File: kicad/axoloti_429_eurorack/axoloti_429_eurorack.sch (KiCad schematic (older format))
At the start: 11 parts, among them J1 SERIAL_SYSTEM_BOOTLOADER, J11 I2C1_HEADER, J30 429_Conn_02x27_Odd_Even_mirro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, J8 429_Conn_02x27_Odd_Even, SW1 BOOT_FLASH, U2 STM32F427IITx

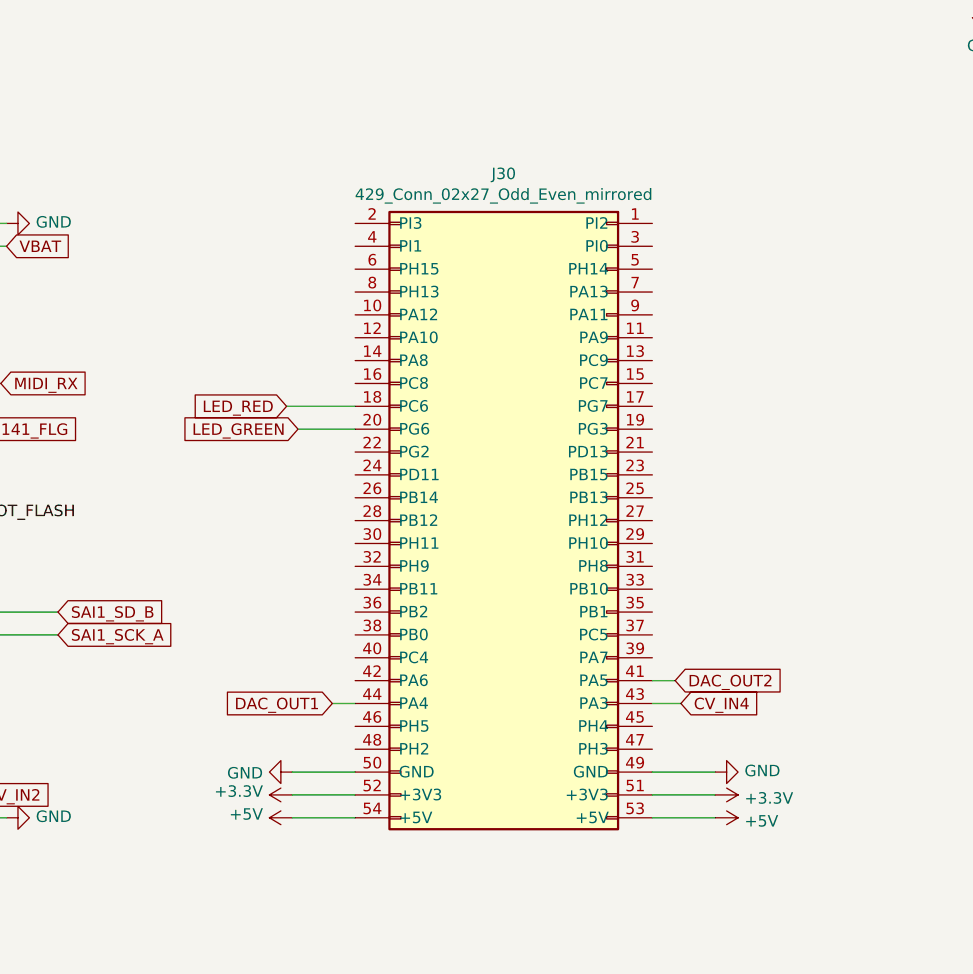
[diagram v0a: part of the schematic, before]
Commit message: create README.md
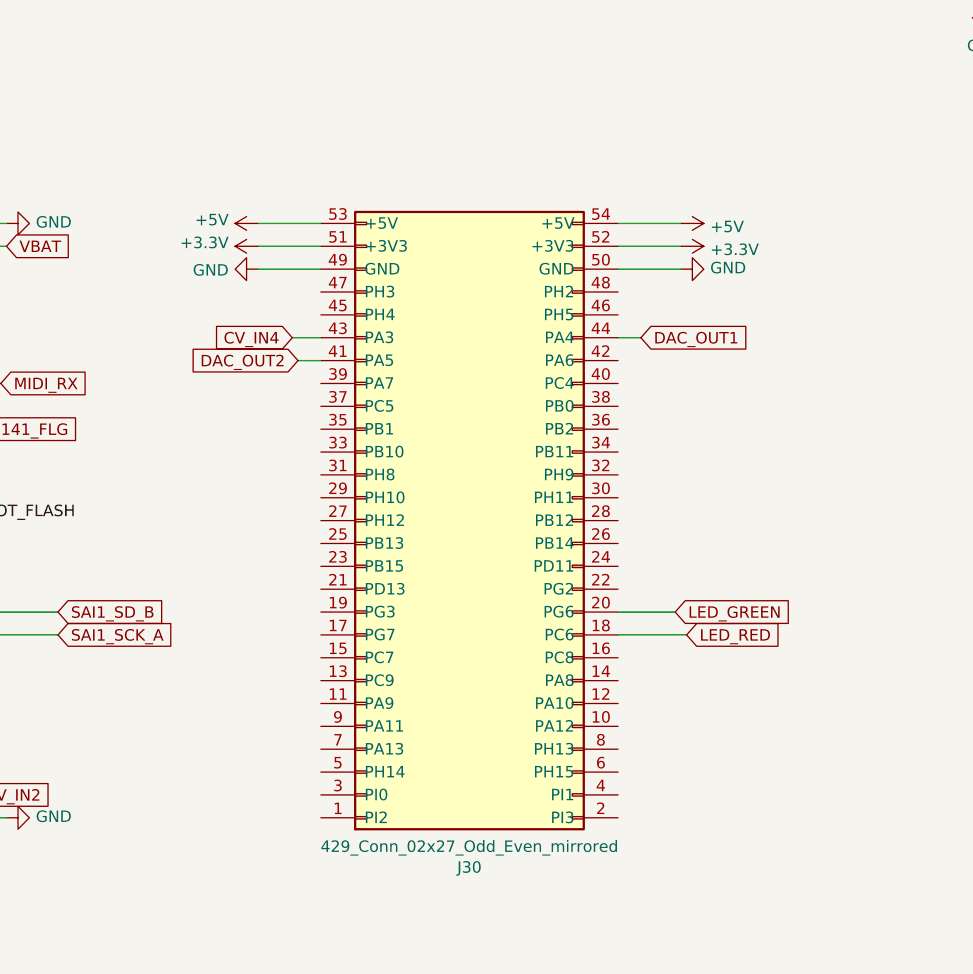
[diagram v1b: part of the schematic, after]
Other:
- moved on the sheet: J30
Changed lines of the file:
@@
 Wire Wire Line
 	12000 6925 11775 6925
-Text GLabel -2200 11800 0    50   Input ~ 0
+Text GLabel -850 10200 2    50   Input ~ 0
 DAC_OUT1
 Wire Wire Line
-	-2200 11800 -2100 11800
-Text GLabel -700 11700 2    50   Input ~ 0
+	-850 10200 -950 10200
+Text GLabel -2350 10300 0    50   Input ~ 0
 DAC_OUT2
 Wire Wire Line
-	-800 11700 -700 11700
+	-2250 10300 -2350 10300
 Text GLabel 11875 2725 2    50   Input ~ 0
 OTG_FS_DM
@@
 Text GLabel -5325 12200 0    50   Input ~ 0
 CV_IN3
-Text GLabel -675 11800 2    50   Input ~ 0
+Text GLabel -2375 10200 0    50   Input ~ 0
 CV_IN4
 Text GLabel 11900 2225 2    50   Input ~ 0
@@
 	-5325 12200 -5200 12200
 Wire Wire Line
-	-800 11800 -675 11800
+	-2250 10200 -2375 10200
 Wire Wire Line
 	11775 2225 11900 2225
@@
 Text Notes 15325 2400 0    50   ~ 0
 done
-Text GLabel -2400 10500 0    50   Input ~ 0
+Text GLabel -650 11500 2    50   Input ~ 0
 LED_RED
 Wire Wire Line
-	-2400 10500 -2100 10500
-Text GLabel -2350 10600 0    50   Input ~ 0
+	-650 11500 -950 11500
+Text GLabel -700 11400 2    50   Input ~ 0
 LED_GREEN
 Wire Wire Line
-	-2350 10600 -2100 10600
+	-700 11400 -950 11400
 Text GLabel 11875 2425 2    50   Input ~ 0
 SAI_MCLK
@@
 L power:GND #PWR0146
 U 1 1 616899AD
-P -2375 12100
-F 0 "#PWR0146" H -2375 11850 50  0001 C CNN
-F 1 "GND" V -2370 11972 50  0000 R CNN
-F 2 "" H -2375 12100 50  0001 C CNN
-F 3 "" H -2375 12100 50  0001 C CNN
-	1    -2375 12100
-	0    1    1    0
-$EndComp
-Wire Wire Line
-	-2375 12100 -2100 12100
+P -675 9900
+F 0 "#PWR0146" H -675 9650 50  0001 C CNN
+F 1 "GND" V -670 9772 50  0000 R CNN
+F 2 "" H -675 9900 50  0001 C CNN
+F 3 "" H -675 9900 50  0001 C CNN
+	1    -675 9900
+	0    -1   -1   0
+$EndComp
+Wire Wire Line
+	-675 9900 -950 9900
 $Comp
 L power:+3.3V #PWR0147
 U 1 1 616BAD54
-P -2375 12200
-F 0 "#PWR0147" H -2375 12050 50  0001 C CNN
-F 1 "+3.3V" V -2360 12328 50  0000 L CNN
-F 2 "" H -2375 12200 50  0001 C CNN
-F 3 "" H -2375 12200 50  0001 C CNN
-	1    -2375 12200
-	0    -1   -1   0
-$EndComp
-Wire Wire Line
-	-2375 12200 -2100 12200
+P -675 9800
+F 0 "#PWR0147" H -675 9650 50  0001 C CNN
+F 1 "+3.3V" V -660 9928 50  0000 L CNN
+F 2 "" H -675 9800 50  0001 C CNN
+F 3 "" H -675 9800 50  0001 C CNN
+	1    -675 9800
+	0    1    1    0
+$EndComp
+Wire Wire Line
+	-675 9800 -950 9800
 $Comp
 L power:+5V #PWR0148
 U 1 1 616EEC4D
-P -2375 12300
-F 0 "#PWR0148" H -2375 12150 50  0001 C CNN
-F 1 "+5V" V -2360 12428 50  0000 L CNN
-F 2 "" H -2375 12300 50  0001 C CNN
-F 3 "" H -2375 12300 50  0001 C CNN
-	1    -2375 12300
-	0    -1   -1   0
-$EndComp
-Wire Wire Line
-	-2375 12300 -2100 12300
+P -675 9700
+F 0 "#PWR0148" H -675 9550 50  0001 C CNN
+F 1 "+5V" V -660 9828 50  0000 L CNN
+F 2 "" H -675 9700 50  0001 C CNN
+F 3 "" H -675 9700 50  0001 C CNN
+	1    -675 9700
+	0    1    1    0
+$EndComp
+Wire Wire Line
+	-675 9700 -950 9700
 Text GLabel -3625 9800 2    50   Input ~ 0
 VBAT
@@
 Wire Wire Line
 	-5475 11800 -5200 11800
-$Comp
-L w_connector:429_Conn_02x27_Odd_Even_mirrored J30
-U 1 1 617A73CC
-P -1450 11000
-F 0 "J30" H -1450 12517 50  0000 C CNN
-F 1 "429_Conn_02x27_Odd_Even_mirrored" H -1450 12426 50  0000 C CNN
-F 2 "" H -1200 11000 50  0001 C CNN
-F 3 "~" H -1200 11000 50  0001 C CNN
-	1    -1450 11000
-	1    0    0    -1
-$EndComp
 Text GLabel -4375 8375 2    50   Input ~ 0
 V_SUPERVIS
@@
 $EndComp
 Wire Wire Line
-	-525 12300 -800 12300
+	-2525 9700 -2250 9700
 $Comp
 L power:+5V #PWR0152
 U 1 1 61707F5F
-P -525 12300
-F 0 "#PWR0152" H -525 12150 50  0001 C CNN
-F 1 "+5V" V -510 12428 50  0000 L CNN
-F 2 "" H -525 12300 50  0001 C CNN
-F 3 "" H -525 12300 50  0001 C CNN
-	1    -525 12300
-	0    1    1    0
-$EndComp
-Wire Wire Line
-	-525 12200 -800 12200
+P -2525 9700
+F 0 "#PWR0152" H -2525 9550 50  0001 C CNN
+F 1 "+5V" V -2510 9828 50  0000 L CNN
+F 2 "" H -2525 9700 50  0001 C CNN
+F 3 "" H -2525 9700 50  0001 C CNN
+	1    -2525 9700
+	0    -1   -1   0
+$EndComp
+Wire Wire Line
+	-2525 9800 -2250 9800
 $Comp
 L power:+3.3V #PWR0151
 U 1 1 616D3BDC
-P -525 12200
-F 0 "#PWR0151" H -525 12050 50  0001 C CNN
-F 1 "+3.3V" V -510 12328 50  0000 L CNN
-F 2 "" H -525 12200 50  0001 C CNN
-F 3 "" H -525 12200 50  0001 C CNN
-	1    -525 12200
-	0    1    1    0
-$EndComp
-Wire Wire Line
-	-525 12100 -800 12100
+P -2525 9800
+F 0 "#PWR0151" H -2525 9650 50  0001 C CNN
+F 1 "+3.3V" V -2510 9928 50  0000 L CNN
+F 2 "" H -2525 9800 50  0001 C CNN
+F 3 "" H -2525 9800 50  0001 C CNN
+	1    -2525 9800
+	0    -1   -1   0
+$EndComp
+Wire Wire Line
+	-2525 9900 -2250 9900
 $Comp
 L power:GND #PWR0150
 U 1 1 616A1448
-P -525 12100
-F 0 "#PWR0150" H -525 11850 50  0001 C CNN
-F 1 "GND" V -520 11972 50  0000 R CNN
-F 2 "" H -525 12100 50  0001 C CNN
-F 3 "" H -525 12100 50  0001 C CNN
-	1    -525 12100
-	0    -1   -1   0
+P -2525 9900
+F 0 "#PWR0150" H -2525 9650 50  0001 C CNN
+F 1 "GND" V -2520 9772 50  0000 R CNN
+F 2 "" H -2525 9900 50  0001 C CNN
+F 3 "" H -2525 9900 50  0001 C CNN
+	1    -2525 9900
+	0    1    1    0
 $EndComp
 Text GLabel -5450 10600 0    50   Input ~ 0
@@
 LCtech already includes 10k pull down
 NoConn ~ -3900 11900
+$Comp
+L w_connector:429_Conn_02x27_Odd_Even_mirrored J30
+U 1 1 617A73CC
+P -1600 11000
+F 0 "J30" H -1600 12517 50  0000 C CNN
+F 1 "429_Conn_02x27_Odd_Even_mirrored" H -1600 12426 50  0000 C CNN
+F 2 "" H -1350 11000 50  0001 C CNN
+F 3 "~" H -1350 11000 50  0001 C CNN
+	1    -1600 11000
+	-1   0    0    1
+$EndComp
 $EndSCHEMATC

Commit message: cleanup
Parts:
- removed U2: STM32F427IITx, LQFP176, symbol w_stm32:STM32F427IITx
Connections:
- wire segments 126 -> 96
- no-connect marks 10 -> 8
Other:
- note added: "I2C pull-ups"
- note removed: "VCC\nGND"
- note removed: "warning: PC13, 14, 15 are weak"
- moved on the sheet: C83, J1, J11, J30, J8, R105, R106, R21, R23, SW1
